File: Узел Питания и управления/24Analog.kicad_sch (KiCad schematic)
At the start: 8 parts

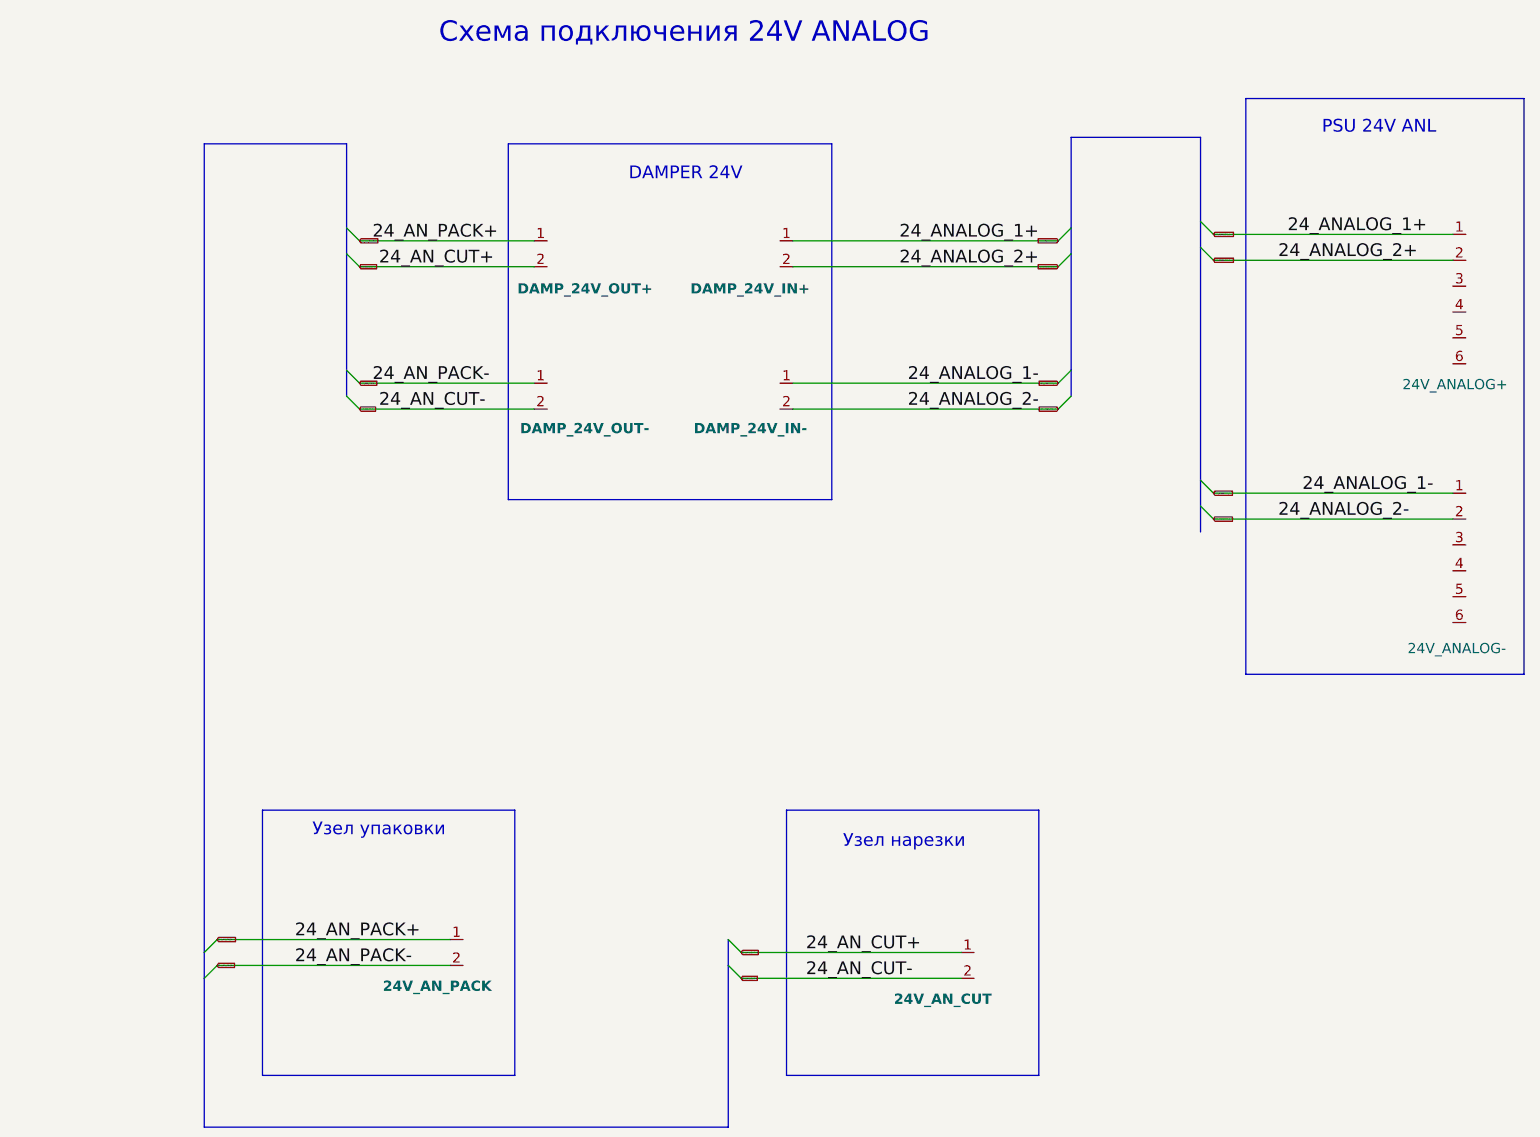
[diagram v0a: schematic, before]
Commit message: update schemas
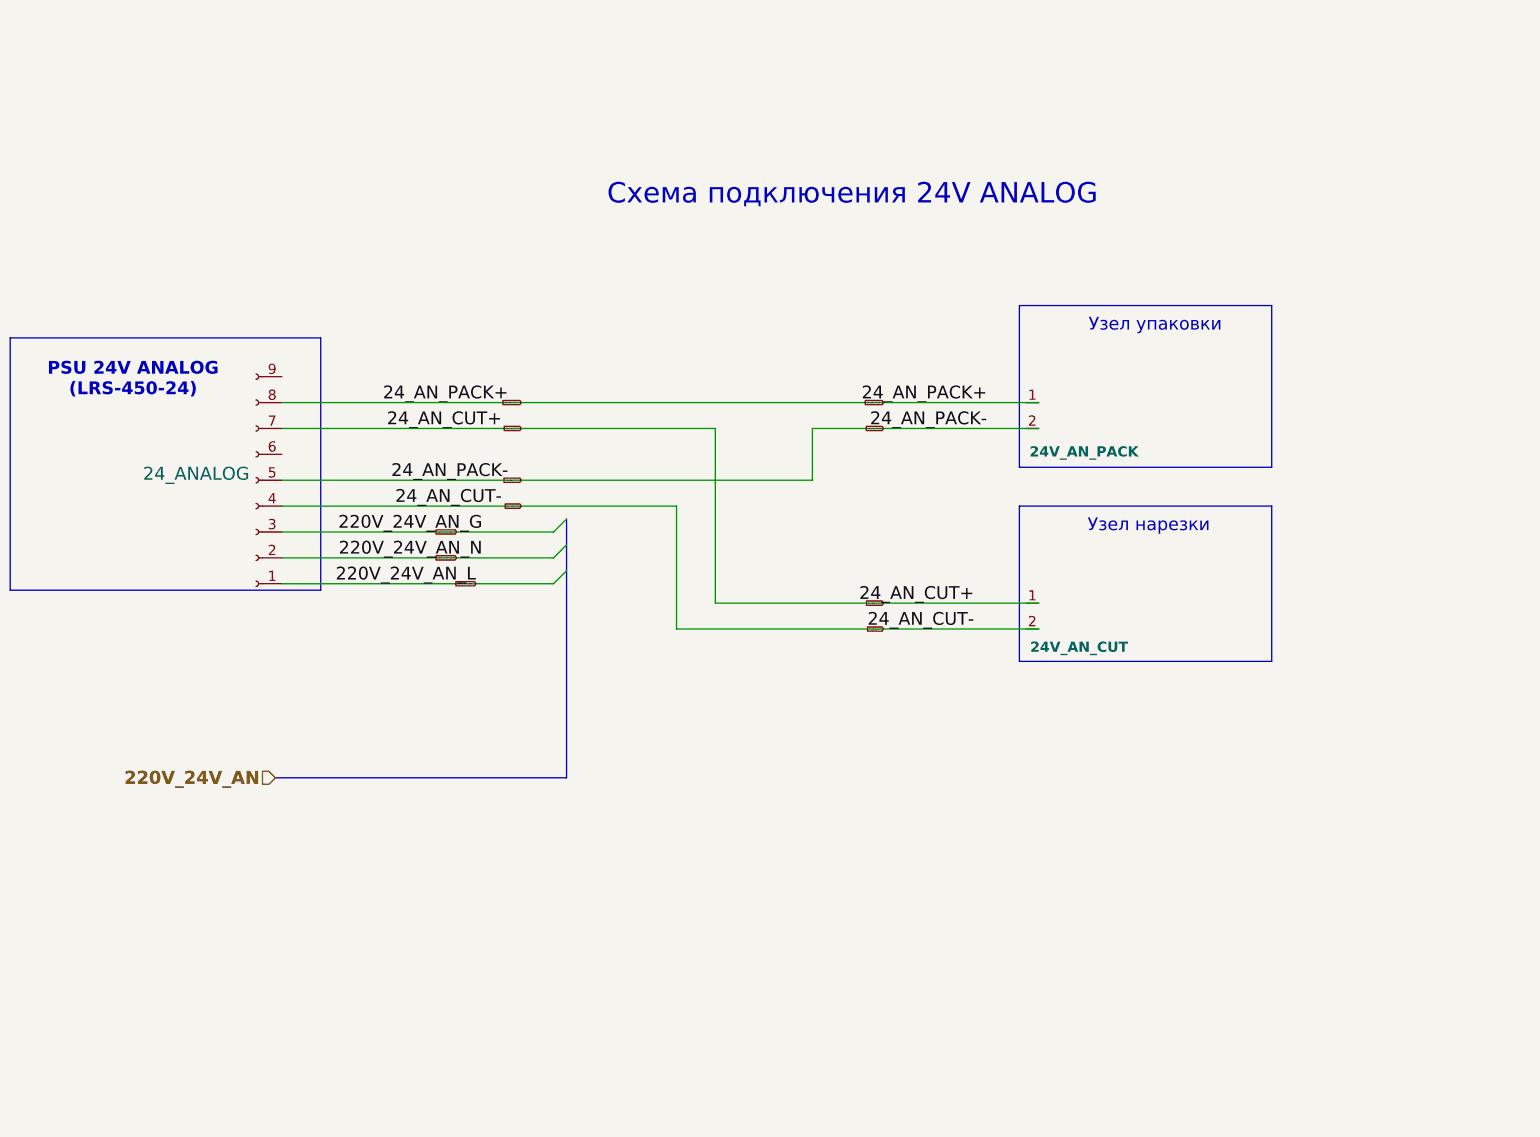
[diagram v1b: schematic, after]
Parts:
- removed 24V_ANALOG+, 24V_ANALOG-: ~, symbol Connector:Conn_01x06_(wide)
- removed DAMP_24V_IN+, DAMP_24V_IN-, DAMP_24V_OUT+, DAMP_24V_OUT-: ~, symbol Connector:Conn_01x02_(wide)
- added J29: 24_ANALOG, symbol Connector:Conn_01x09_Socket_WIDE
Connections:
- net 24_AN_CUT+: now also J29.7 (Pin_7)
- net 24_AN_CUT-: now also J29.4 (Pin_4)
- net 24_AN_PACK+: now also J29.8 (Pin_8)
- net 24_AN_PACK-: now also J29.5 (Pin_5)
- new net 220V_24V_AN_G: J29.3 (Pin_3)
- new net 220V_24V_AN_L: J29.1 (Pin_1)
- new net 220V_24V_AN_N: J29.2 (Pin_2)
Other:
- note added: "PSU 24V ANALOG (LRS-450-24)"
- note removed: "DAMPER 24V"
- note removed: "PSU 24V ANL"
- moved on the sheet: 24V_AN_CUT, 24V_AN_PACK
